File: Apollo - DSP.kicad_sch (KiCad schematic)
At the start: 27 parts, among them J1 USB_C_Receptacle_USB2.0, U1 NCP115ASN330T2G, U2 NCP115ASN330T2G, U3 USBLC6-2SC6

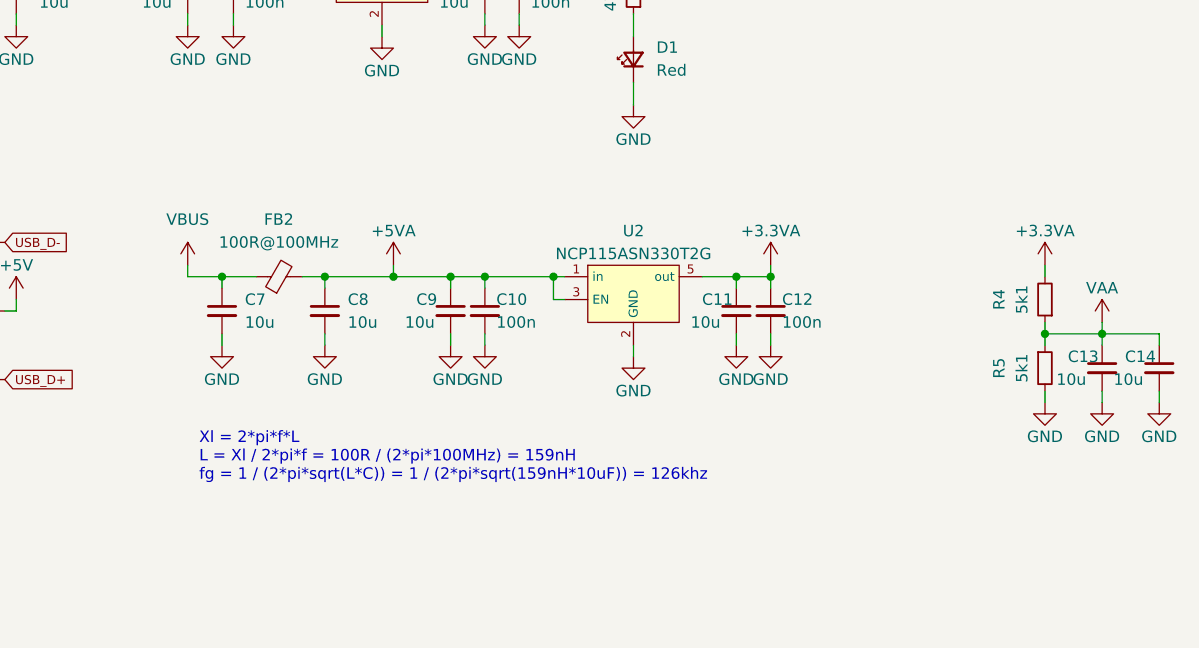
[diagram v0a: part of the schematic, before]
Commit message: modifications for rev 3
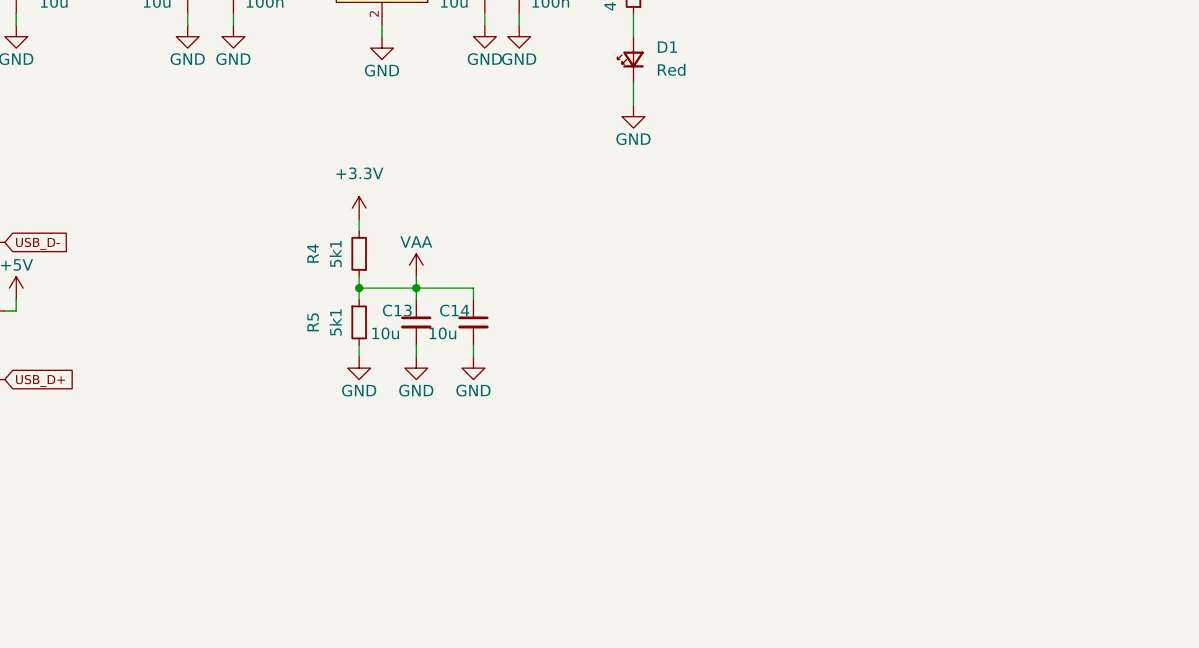
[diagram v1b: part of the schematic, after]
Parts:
- removed C10, C12: 100n, Capacitor_SMD:C_0603_1608Metric_Pad1.08x0.95mm_HandSolder, symbol Device:C_Small
- removed C11, C7, C8, C9: 10u, Capacitor_SMD:C_0603_1608Metric_Pad1.08x0.95mm_HandSolder, symbol Device:C_Small
- removed FB2: 100R@100MHz, Resistor_SMD:R_0603_1608Metric_Pad0.98x0.95mm_HandSolder, symbol Device:FerriteBead_Small
- removed U2: NCP115ASN330T2G, NCP115ASN330T2G:NCP115ASN330T2G, symbol NCP115ASN330T2G:NCP115ASN330T2G
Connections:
- net +3.3VA is gone; now on net +3V3: R4.2
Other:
- moved on the sheet: C13, C14, R4, R5
